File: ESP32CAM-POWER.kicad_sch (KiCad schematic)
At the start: 22 parts, among them J1 Conn_01x02_Female, J2 Conn_01x06_Male, J3 Conn_01x02_Male, SW1 BOOT, U1 D-SUN-MP1584EN, U2 ESP32-CAM

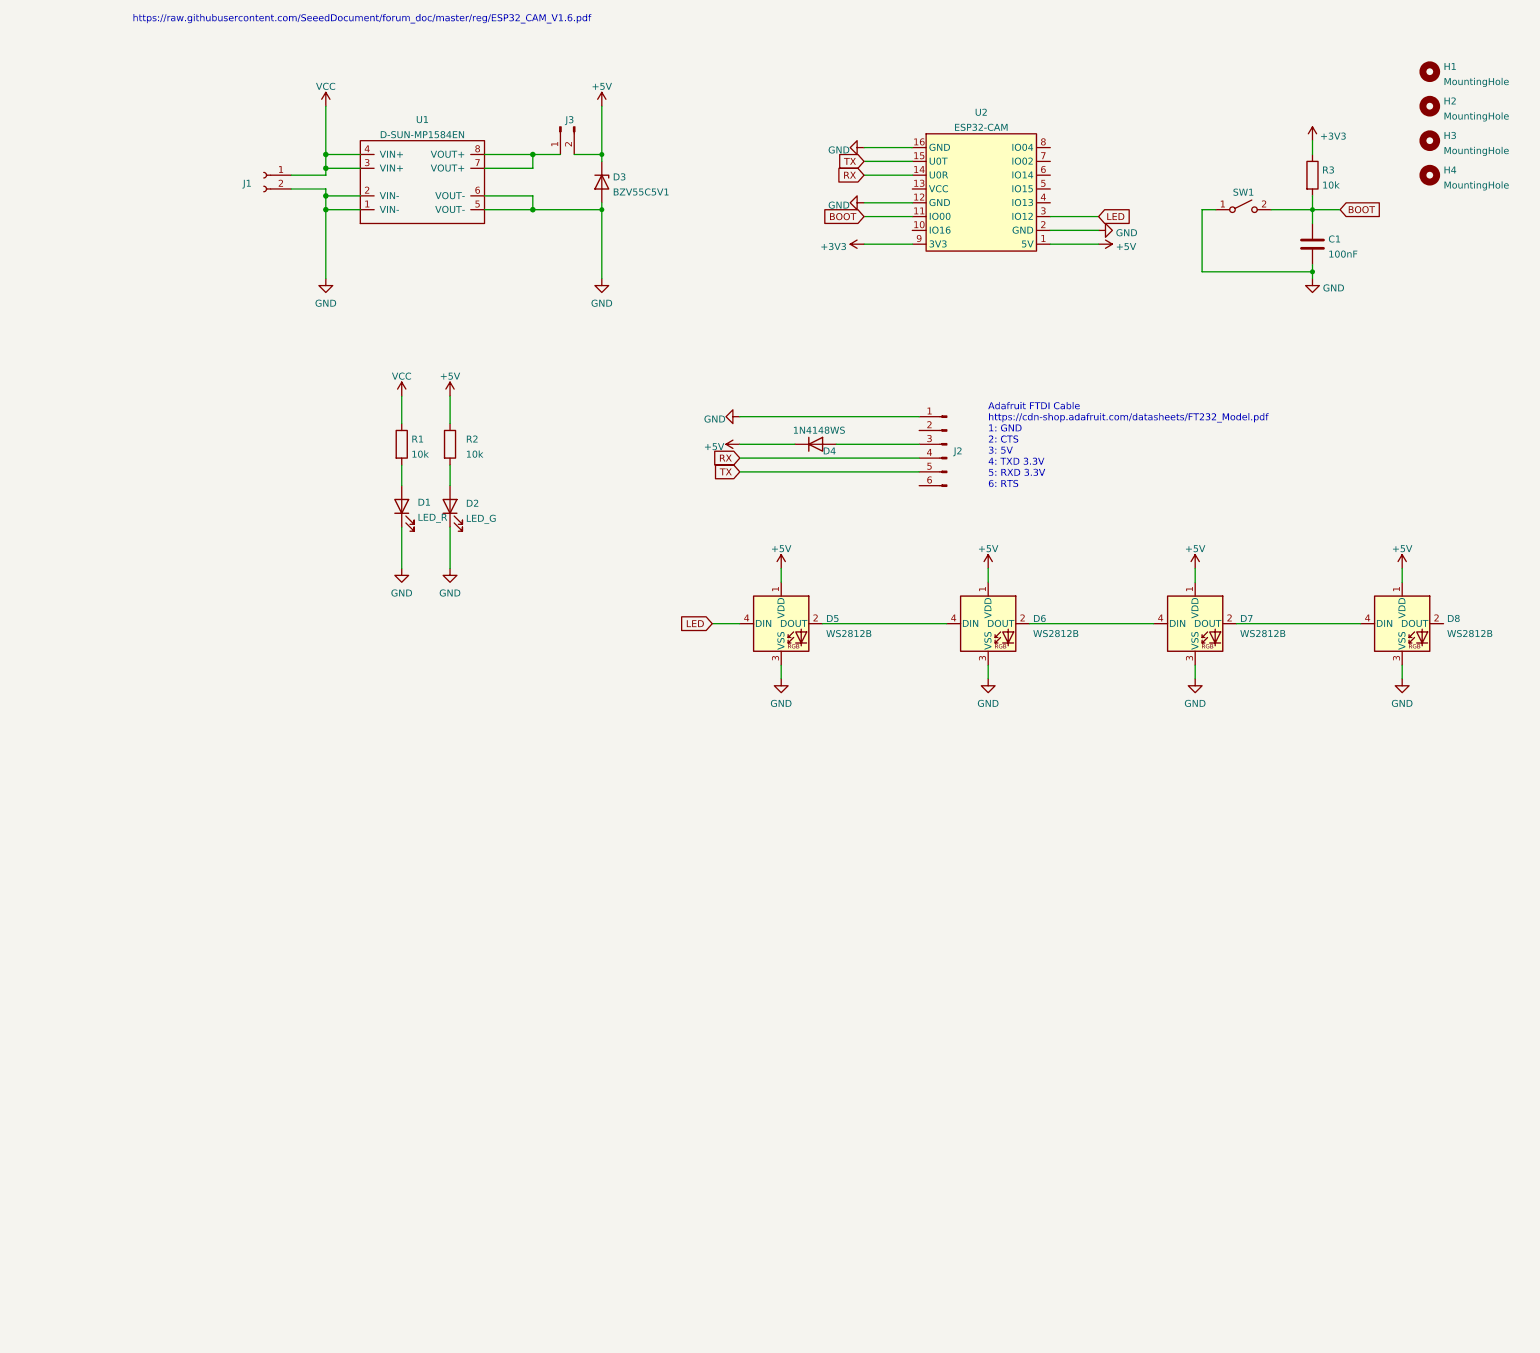
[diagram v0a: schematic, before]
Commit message: serveral changes, add USB, still a bit messy
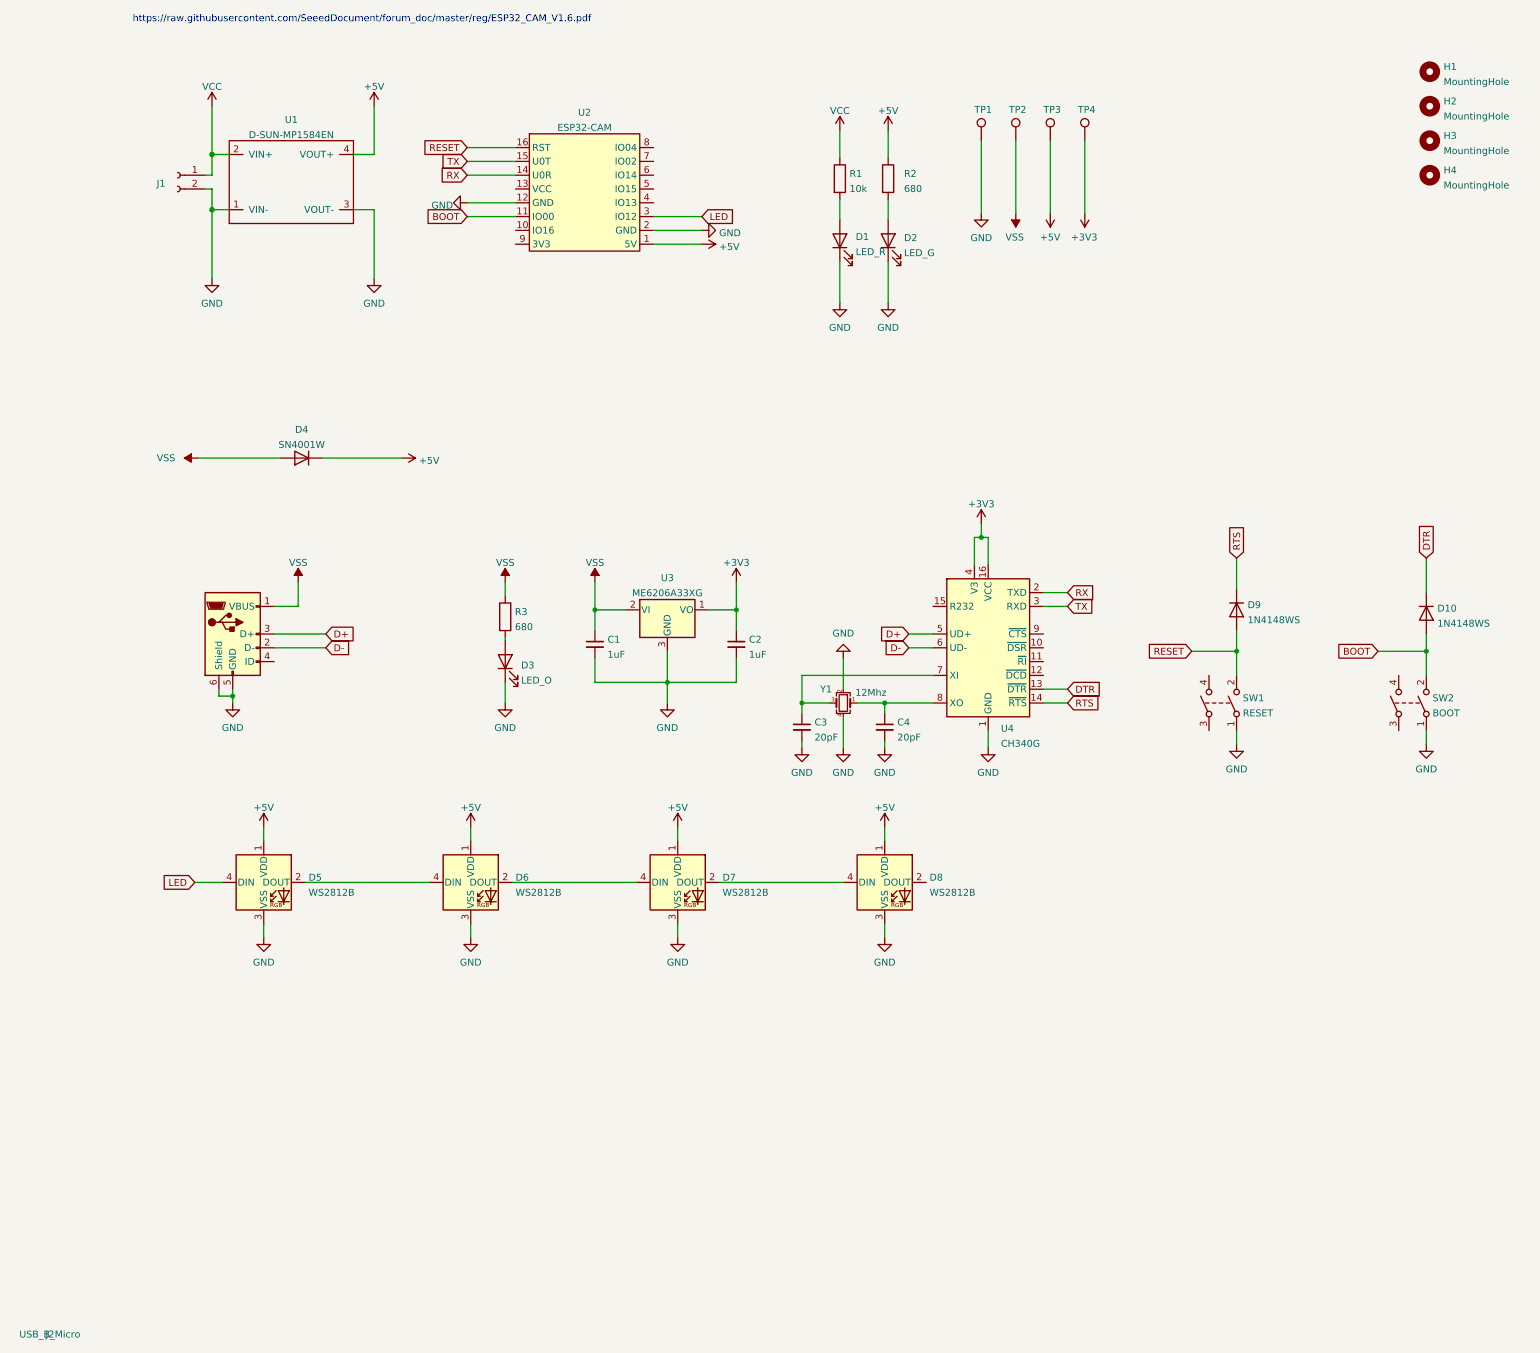
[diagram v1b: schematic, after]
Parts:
- removed C1: 100nF, Capacitor_SMD:C_0603_1608Metric, symbol Device:C
- removed D3: BZV55C5V1, Diode_SMD:D_MiniMELF, symbol Diode:BZV55C5V1
- removed D4: 1N4148WS, Diode_SMD:D_SOD-323, symbol Diode:1N4148WS
- removed J2: Conn_01x06_Male, Connector_PinHeader_2.54mm:PinHeader_1x06_P2.54mm_Horizontal, symbol Connector:Conn_01x06_Male
- removed J3: Conn_01x02_Male, Jumper:SolderJumper-2_P1.3mm_Open_RoundedPad1.0x1.5mm, symbol Connector:Conn_01x02_Male
- removed SW1: BOOT, Button_Switch_SMD:SW_Push_1P1T_NO_6x6mm_H9.5mm, symbol Switch:SW_SPST
- added C1, C2: 1uF, Capacitor_SMD:C_0603_1608Metric, symbol Device:C_Small
- added C3, C4: 20pF, Capacitor_SMD:C_0603_1608Metric, symbol Device:C_Small
- added D10, D9: 1N4148WS, Diode_SMD:D_SOD-323, symbol Diode:1N4148WS
- added D3: LED_O, LED_SMD:LED_0603_1608Metric, symbol Device:LED
- added D4: SN4001W, Diode_SMD:D_SOD-123, symbol Diode:SM4001
- added J2: USB_B_Micro, Connector_USB:USB_Micro-B_Amphenol_10118194_Horizontal, symbol Connector:USB_B_Micro
- added SW1: RESET, bouni:TS-1187A-B-A-B, symbol Switch:SW_DPST
- added SW2: BOOT, bouni:TS-1187A-B-A-B, symbol Switch:SW_DPST
- added TP1, TP2, TP3, TP4: TestPoint, TestPoint:TestPoint_Pad_D1.5mm, symbol Connector:TestPoint
- added U3: ME6206A33XG, Package_TO_SOT_SMD:SOT-23, symbol Regulator_Linear:LM3480-3.3
- added U4: CH340G, Package_SO:SOIC-16_3.9x9.9mm_P1.27mm, symbol Interface_USB:CH340G
- added Y1: 12Mhz, Crystal:Crystal_SMD_3225-4Pin_3.2x2.5mm, symbol Device:Crystal_GND24_Small
- D5, D6, D7, D8, H1, H2, H3, H4, U1, U2: now left out of the parts list
- J1: footprint Connector_Phoenix_MSTB:PhoenixContact_MSTBVA_2,5_2-G-5,08_1x02_P5.08mm_Vertical -> TerminalBlock_RND:TerminalBlock_RND_205-00232_1x02_P5.08mm_Horizontal; now left out of the parts list
- R2, R3: value 10k -> 680
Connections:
- net +3V3: now also C2.1, TP4.1, U3.1 (VO), U4.16 (VCC), U4.4 (V3); no longer R3.1, U2.9 (3V3)
- net +5V: now also U1.4 (VOUT+), D4.1 (K), TP3.1
- net BOOT: now also D10.2 (A), SW2.2; no longer R3.2
- net GND: now also U1.3 (VOUT-), C1.2, C2.2, C3.2, C4.2, D3.1 (K), J2.5 (GND), J2.6 (Shield), SW1.1, SW2.1, TP1.1, U3.3 (GND), U4.1 (GND), Y1.2, Y1.4; no longer U1.2 (VIN-), U1.5 (VOUT-), U1.6 (VOUT-), U2.16 (GND)
- net RX: now also U4.2 (TXD)
- net TX: now also U4.3 (RXD)
- net VCC: now also U1.2 (VIN+); no longer U1.3 (VIN+), U1.4 (VIN+)
- new net: D3.2 (A), R3.2
- new net: C3.1, U4.7 (XI), Y1.3
- new net: C4.1, U4.8 (XO), Y1.1
- new net D+: J2.3 (D+), U4.5 (UD+)
- new net D-: J2.2 (D-), U4.6 (UD-)
- new net DTR: D10.1 (K), U4.13 (~{DTR})
- new net RESET: D9.2 (A), SW1.2, U2.16 (RST)
- new net RTS: D9.1 (K), U4.14 (~{RTS})
- new net VSS: C1.1, D4.2 (A), J2.1 (VBUS), R3.1, TP2.1, U3.2 (VI)
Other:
- note removed: "Adafruit FTDI Cable https://cdn-shop.adafruit.com/datasheets/FT232_Model.pdf 1: GND 2: CTS 3: 5V 4: TXD 3.3V 5: RXD 3.3V 6: RTS"
- moved on the sheet: D1, D2, D5, D6, D7, D8, J1, R1, R2, U2
